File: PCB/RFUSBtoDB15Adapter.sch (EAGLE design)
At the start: 7 parts, among them J2 AVR_SPI_PROG_3X2NS

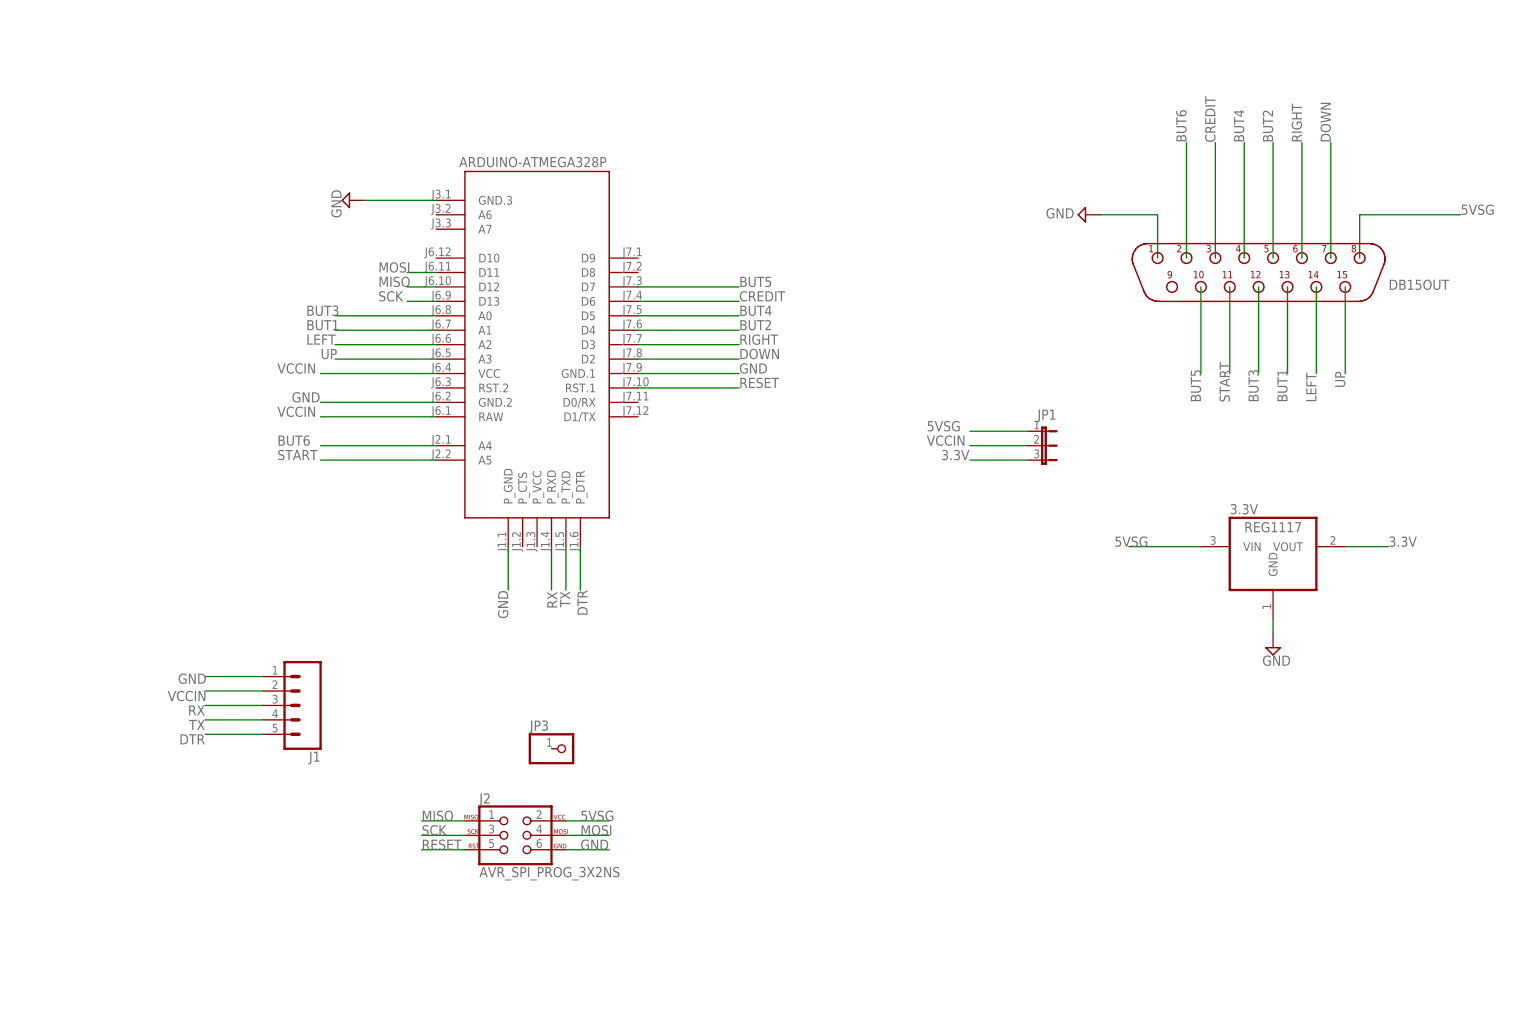
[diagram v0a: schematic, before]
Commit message: New PCB
PCB updated
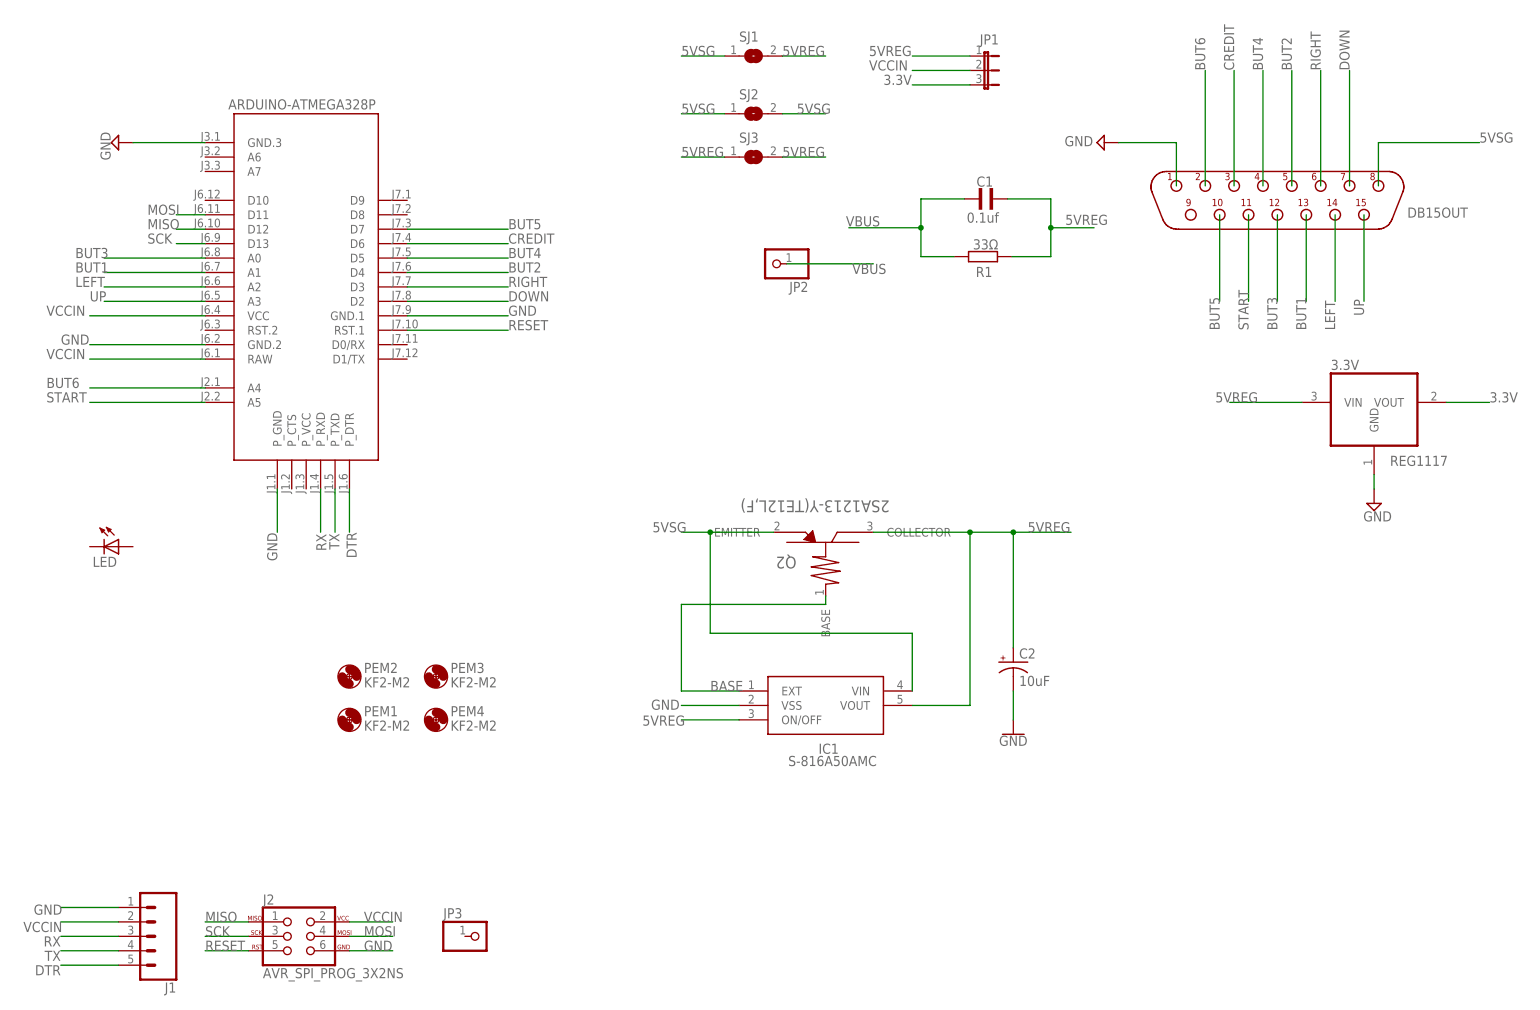
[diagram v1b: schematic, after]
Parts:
- added C1: 0.1uf, Wurth_Elektronik_Passive_Capacitors_rev18b:WCAP-CSGP_0805_885012006082_REFLOW
- added C2: 10uF, SparkFun-Capacitors:10UF-POLAR-EIA3216-16V-10%(TANT)
- added IC1: S-816A40AMC-BAPT2U, S-816A40AMC-BAPT2U:S-816A40AMC-BAPT2U
- added JP2: (no value), pinhead:PINHD-1X1
- added LED: (no value), adafruit:LED3MM
- added PEM1, PEM2, PEM3, PEM4: KF2-M2, penn-engineering:KF2-M2
- added Q2: 2SA1213-Y(TE12L,F), 2SA1213YTE12LF:2SA1213-Y(TE12L,F)
- added R1: 33Ω, eagle-ltspice:R
- added SJ1, SJ2, SJ3: (no value), jumper:SJ
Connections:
- new net 5VREG: 3.3V.VIN, C1.1, C2.+, IC1.ON/OFF, IC1.VOUT, JP1.1, Q2.COLLECTOR, R1.2, SJ1.2, SJ3.1, SJ3.2
- new net BASE: IC1.EXT, Q2.BASE
- new net VBUS: C1.2, JP2.1, R1.1
- net 5VSG: now also IC1.VIN, Q2.EMITTER, SJ1.1, SJ2.1, SJ2.2; no longer 3.3V.VIN, J2.2, JP1.1
- net GND: now also C2.-, IC1.VSS
- net VCCIN: now also J2.2
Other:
- note added: "IF USING A 5V ARDUINO, FEED RAW (VCCIN) PIN WITH 3.3V FROM THE REGULATOR (REG1117)."
- note added: "THE 5V REGULATOR (IC1) WILL PROTECT THE VCC LINE FROM A POSSIBLE BAD PSU VOLTAGE, IF YOU DON'T NEED, JUST JUMPER SJ1."
- note removed: "IF USING A 5V ARDUINO, FEED RAW WITH 3.3V FROM THE REGULATOR."
- moved on the sheet: 3.3V, ARDUINO-ATMEGA328P, DB15OUT, J1, J2, JP1, JP3
